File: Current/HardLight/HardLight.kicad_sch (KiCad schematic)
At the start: 47 parts, among them J0 USB, J1 qwiic, J2 MicroCon, J3 MicroCon, U0 RP2040, U1 LDO-3.3, U2 USBLC6-2SC6, U3 W25Q128JVS, Y0 2TJ412000NYGBC 12MHz

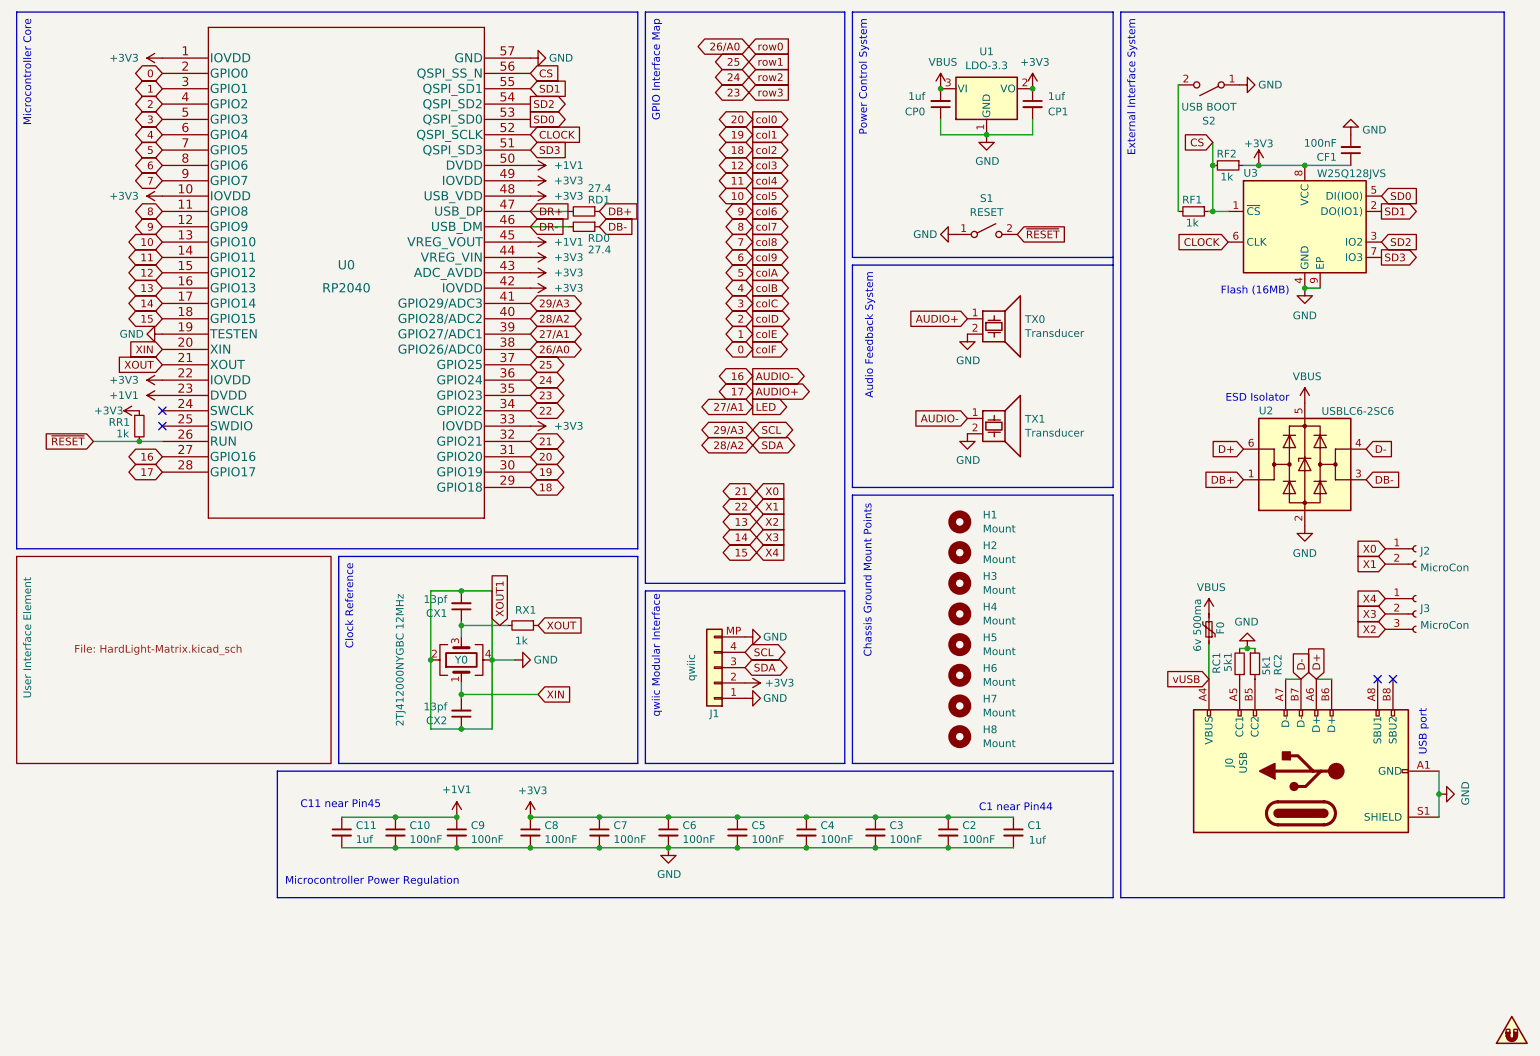
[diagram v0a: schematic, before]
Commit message: So much stuff
Wow it's been a while.
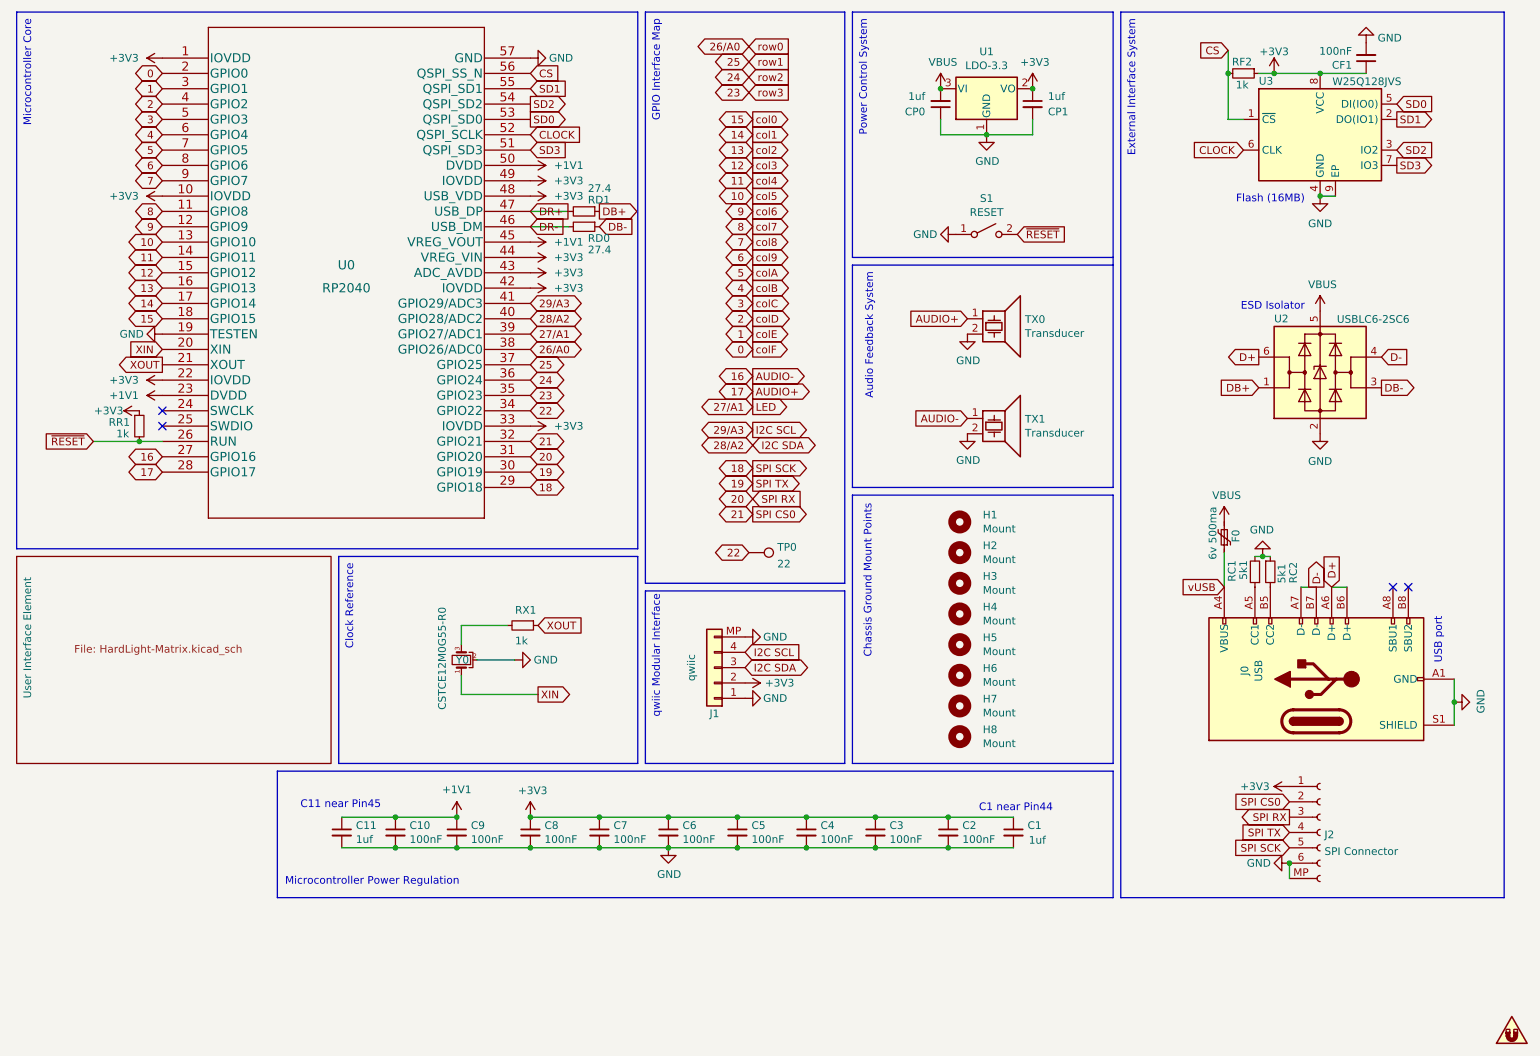
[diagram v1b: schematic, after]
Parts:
- removed CX1, CX2: 13pf, EDI:Passive_0402_1005Metric, symbol Device:C_Small
- removed J2: MicroCon, EDI:MicroCon-2, symbol Connector:Conn_01x02_Female
- removed J3: MicroCon, EDI:MicroCon-3, symbol Connector:Conn_01x03_Female
- removed RF1: 1k, EDI:Passive_0402_1005Metric, symbol Device:R_Small
- removed S2: USB BOOT, Button_Switch_SMD:SW_SPST_SKQG_WithoutStem, symbol Switch:SW_SPST
- removed Y0: 2TJ412000NYGBC 12MHz, Crystal:Crystal_SMD_2520-4Pin_2.5x2.0mm, symbol Device:Crystal_GND24
- added J2: SPI Connector, Connector_JST:JST_SH_SM06B-SRSS-TB_1x06-1MP_P1.00mm_Horizontal, symbol Connector:Conn_01x07_Female
- added TP0: 22, TestPoint:TestPoint_Pad_1.0x1.0mm, symbol Connector:TestPoint
- added Y0: CSTCE12M0G55-R0, Crystal:Resonator_SMD_Murata_CSTxExxV-3Pin_3.0x1.1mm, symbol Device:Crystal_GND2_Small
- F0: footprint Fuse:Fuse_0603_1608Metric -> Fuse:Fuse_0402_1005Metric; LCSC C207011 -> C206938
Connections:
- net +3V3: now also J2.1 (Pin_1)
- net 18: now also J2.5 (Pin_5)
- net 19: now also J2.4 (Pin_4)
- net 20: now also J2.3 (Pin_3)
- net 21: now also J2.2 (Pin_2)
- net 22: now also TP0.1
- net GND: now also J2.6 (Pin_6), J2.MP, Y0.2
- net XIN: now also Y0.1
- net XOUT1: no longer names the net of RX1.2
- net XOUT1: now also Y0.3
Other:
- moved on the sheet: CF1, F0, J0, RC1, RC2, RF2, U2, U3
